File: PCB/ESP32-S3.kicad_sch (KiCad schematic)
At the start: 5 parts, among them J1 USB_C_Receptacle_USB2.0_16P

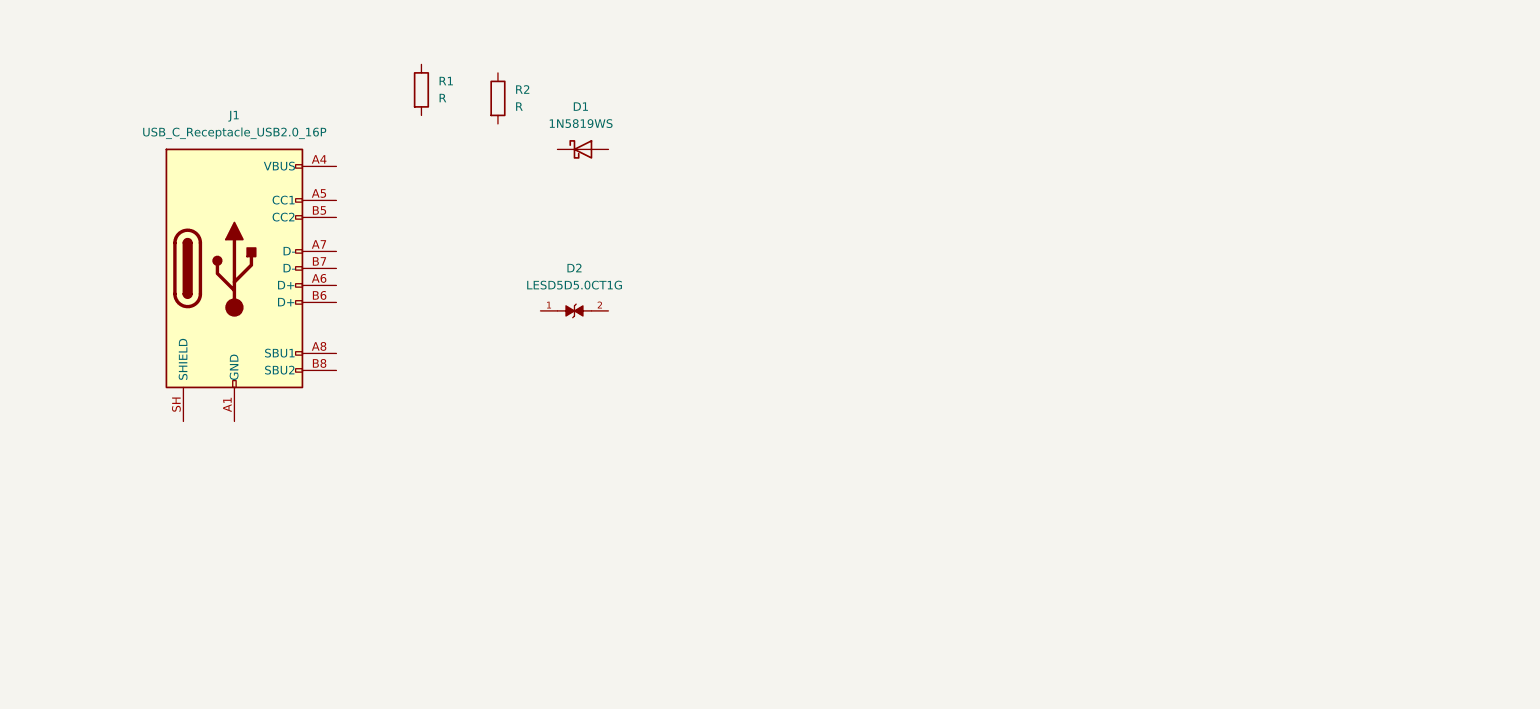
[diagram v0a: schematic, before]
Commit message: [Schem] Uhh made the Amplifier & motor driver circuits
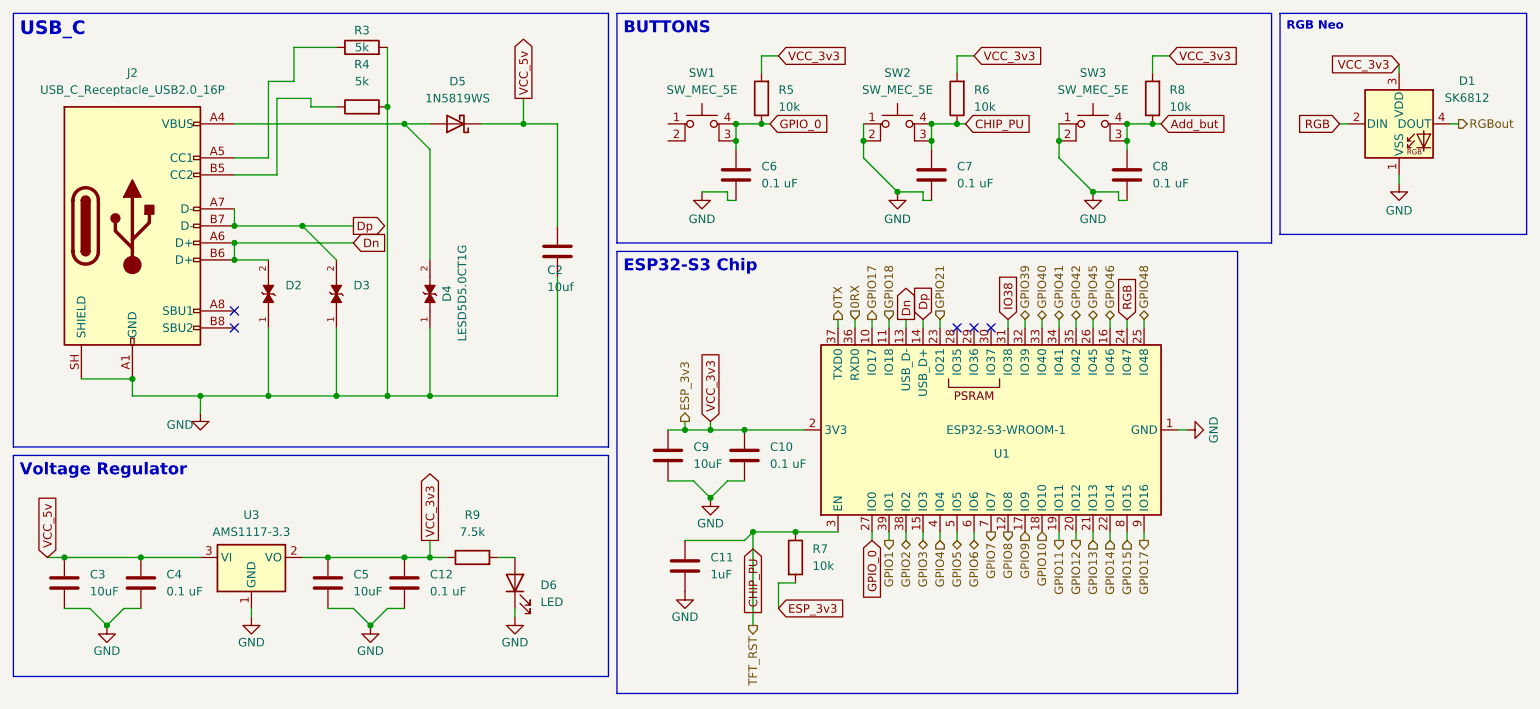
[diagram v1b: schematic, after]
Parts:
- removed D1: 1N5819WS, Diode_SMD:D_SOD-323, symbol Diode:1N5819WS
- removed D2: LESD5D5.0CT1G, LESD5D5.0CT1G:TVS_LESD5D5.0CT1G, symbol WALL-E_SYM:LESD5D5.0CT1G
- removed J1: USB_C_Receptacle_USB2.0_16P, symbol Connector:USB_C_Receptacle_USB2.0_16P
- removed R1, R2: R, symbol Device:R
- added C10, C12, C4, C6, C7, C8: 0.1 uF, Capacitor_SMD:C_0603_1608Metric_Pad1.08x0.95mm_HandSolder, symbol Device:C
- added C11: 1uF, Capacitor_SMD:C_0603_1608Metric_Pad1.08x0.95mm_HandSolder, symbol Device:C
- added C2: 10uf, Capacitor_SMD:C_0603_1608Metric_Pad1.08x0.95mm_HandSolder, symbol Device:C
- added C3, C5, C9: 10uF, Capacitor_SMD:C_0603_1608Metric_Pad1.08x0.95mm_HandSolder, symbol Device:C
- added D1: SK6812, LED_SMD:LED_SK6812_PLCC4_5.0x5.0mm_P3.2mm, symbol LED:SK6812
- added D2, D3, D4: LESD5D5.0CT1G, LESD5D5.0CT1G:TVS_LESD5D5.0CT1G, symbol WALL-E_symbols:LESD5D5.0CT1G
- added D5: 1N5819WS, Diode_SMD:D_SOD-323, symbol Diode:1N5819WS
- added D6: LED, LED_SMD:LED_0603_1608Metric_Pad1.05x0.95mm_HandSolder, symbol Device:LED
- added J2: USB_C_Receptacle_USB2.0_16P, Connector_USB:USB_C_Receptacle_Amphenol_12401610E4-2A_CircularHoles, symbol Connector:USB_C_Receptacle_USB2.0_16P
- added R3, R4: 5k, Resistor_SMD:R_0603_1608Metric_Pad0.98x0.95mm_HandSolder, symbol Device:R
- added R5, R6, R7, R8: 10k, Resistor_SMD:R_0603_1608Metric_Pad0.98x0.95mm_HandSolder, symbol Device:R
- added R9: 7.5k, Resistor_SMD:R_0603_1608Metric_Pad0.98x0.95mm_HandSolder, symbol Device:R
- added SW1, SW2, SW3: SW_MEC_5E, RAM:SW_Push_1P1T_NO_CK_KMR2, symbol Switch:SW_MEC_5E
- added U1: ESP32-S3-WROOM-1, RF_Module:ESP32-S3-WROOM-1, symbol RF_Module:ESP32-S3-WROOM-1
- added U3: AMS1117-3.3, Package_TO_SOT_SMD:SOT-223-3_TabPin2, symbol Regulator_Linear:AMS1117-3.3
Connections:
- new net: D6.2 (A), R9.2
- new net: D4.2, D5.2 (A), J2.A4 (VBUS), J2.A9 (VBUS), J2.B4 (VBUS), J2.B9 (VBUS)
- new net: J2.A5 (CC1), R3.1
- new net: J2.B5 (CC2), R4.1
- new net 0RX: U1.36 (RXD0)
- new net 0TX: U1.37 (TXD0)
- new net Add_but: C8.1, R8.1, SW3.3 (K), SW3.4 (A)
- new net CHIP_PU: C11.1, C7.1, R6.1, R7.1, SW2.3 (K), SW2.4 (A), U1.3 (EN)
- new net Dn: D2.2, J2.A6 (D+), J2.B6 (D+), U1.13 (USB_D-)
- new net Dp: D3.2, J2.A7 (D-), J2.B7 (D-), U1.14 (USB_D+)
- new net ESP_3v3: C10.1, C12.1, C5.1, C9.1, D1.3 (VDD), R5.2, R6.2, R7.2, R8.2, R9.1, U1.2 (3V3), U3.2 (VO)
- new net GND: C10.2, C11.2, C12.2, C2.2, C3.2, C4.2, C5.2, C6.2, C7.2, C8.2, C9.2, D1.1 (VSS), D2.1, D3.1, D4.1, D6.1 (K), J2.A1 (GND), J2.A12 (GND), J2.B1 (GND), J2.B12 (GND), J2.SH (SHIELD), R3.2, R4.2, SW2.1, SW2.2, SW3.1, SW3.2, U1.1 (GND), U1.40 (GND), U1.41 (GND), U3.1 (GND)
- new net GPIO1: U1.39 (IO1)
- new net GPIO10: U1.18 (IO10)
- new net GPIO11: U1.19 (IO11)
- new net GPIO12: U1.20 (IO12)
- new net GPIO13: U1.21 (IO13)
- new net GPIO14: U1.22 (IO14)
- new net GPIO15: U1.8 (IO15)
- new net GPIO17: U1.10 (IO17), U1.9 (IO16)
- new net GPIO18: U1.11 (IO18)
- new net GPIO2: U1.38 (IO2)
- new net GPIO21: U1.23 (IO21)
- new net GPIO3: U1.15 (IO3)
- new net GPIO39: U1.32 (IO39)
- new net GPIO4: U1.4 (IO4)
- new net GPIO40: U1.33 (IO40)
- new net GPIO41: U1.34 (IO41)
- new net GPIO42: U1.35 (IO42)
- new net GPIO45: U1.26 (IO45)
- new net GPIO46: U1.16 (IO46)
- new net GPIO48: U1.25 (IO48)
- new net GPIO5: U1.5 (IO5)
- new net GPIO6: U1.6 (IO6)
- new net GPIO7: U1.7 (IO7)
- new net GPIO8: U1.12 (IO8)
- new net GPIO9: U1.17 (IO9)
- new net GPIO_0: C6.1, R5.1, SW1.3 (K), SW1.4 (A), U1.27 (IO0)
- new net IO38: U1.31 (IO38)
- new net RGB: D1.2 (DIN), U1.24 (IO47)
- new net RGBout: D1.4 (DOUT)
- new net VCC_5v: C2.1, C3.1, C4.1, D5.1 (K), U3.3 (VI)
- no-connect marks 0 -> 5
